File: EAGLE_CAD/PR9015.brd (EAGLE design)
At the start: 70 x 70 mm, 73 parts, among them J1 M3_SCREW_POST, SW1 C&K_PTS645

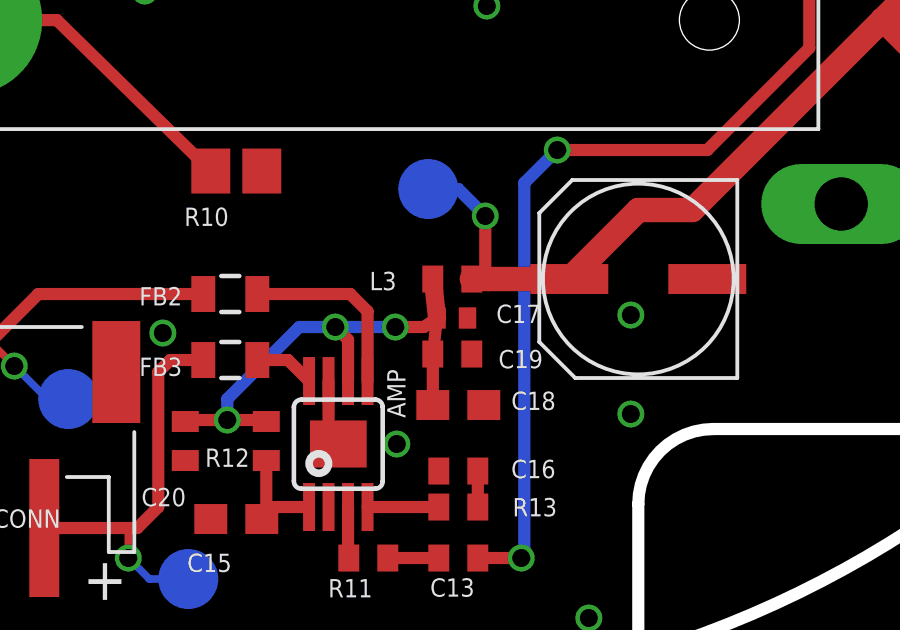
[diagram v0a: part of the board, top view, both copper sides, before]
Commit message: Revert cea9e40..4e97d22
This rolls back to commit cea9e40d509ff5bb8dd7e4369702d55ec1f1bc0f.
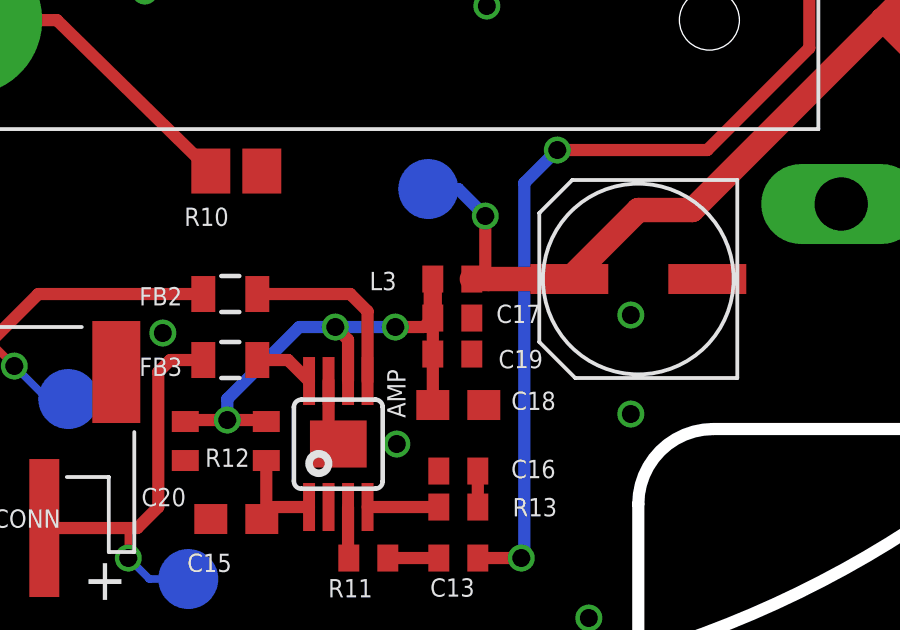
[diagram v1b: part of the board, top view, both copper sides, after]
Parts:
- C17: device PR_Parts_Library:C0402 -> resistor:C0402
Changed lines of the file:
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@@
 <?xml version="1.0" encoding="utf-8"?>
 <!DOCTYPE eagle SYSTEM "eagle.dtd">
-<eagle version="6.6.0">
+<eagle version="7.2.0">
 <drawing>
 <settings>
@@
 <setting verticaltext="up"/>
 </settings>
-<grid distance="0.1" unitdist="mm" unit="mm" style="lines" multiple="1" display="yes" altdistance="0.025" altunitdist="inch" altunit="inch"/>
+<grid distance="1" unitdist="mil" unit="mm" style="lines" multiple="1" display="yes" altdistance="0.025" altunitdist="inch" altunit="inch"/>
 <layers>
 <layer number="1" name="Top" color="4" fill="1" visible="yes" active="yes"/>
@@
 <pass name="Default">
 <param name="RoutingGrid" value="50mil"/>
+<param name="AutoGrid" value="1"/>
+<param name="Efforts" value="0"/>
+<param name="TopRouterVariant" value="1"/>
 <param name="tpViaShape" value="round"/>
 <param name="PrefDir.1" value="|"/>
@@
 <attribute name="VALUE" x="32.235" y="7.905" size="1.27" layer="27" rot="R180"/>
 </element>
-<element name="C17" library="PR_Parts_Library" package="C0402" value="1uf" x="38.8" y="12.7" smashed="yes" rot="R180">
+<element name="C17" library="resistor" package="C0402" value="1uf" x="38.8" y="12.7" smashed="yes" rot="R180">
 <attribute name="NAME" x="40.265" y="12.535" size="0.6096" layer="25" ratio="16"/>
 <attribute name="VALUE" x="39.435" y="14.605" size="1.27" layer="27" rot="R180"/>
@@
 <wire x1="34.9" y1="12.4" x2="33.7" y2="12.4" width="0.4064" layer="16"/>
 <wire x1="33.7" y1="12.4" x2="31.3" y2="10" width="0.4064" layer="16"/>
-<wire x1="38.2929" y1="12.7" x2="37.85" y2="12.4" width="0.4064" layer="1"/>
+<wire x1="38.15" y1="12.7" x2="37.85" y2="12.4" width="0.4064" layer="1"/>
 <wire x1="37.85" y1="12.4" x2="36.9" y2="12.4" width="0.4064" layer="1"/>
 <via x="36.9" y="12.4" extent="1-16" drill="0.6"/>
 <wire x1="36.9" y1="12.4" x2="34.9" y2="12.4" width="0.4064" layer="16"/>
 <wire x1="38.15" y1="9.8" x2="38.15" y2="11.5" width="0.4064" layer="1"/>
-<wire x1="38.15" y1="11.5" x2="38.2929" y2="12.7" width="0.4064" layer="1"/>
+<wire x1="38.15" y1="11.5" x2="38.15" y2="12.7" width="0.4064" layer="1"/>
 <wire x1="31.3" y1="10" x2="31.3" y2="9.3" width="0.4064" layer="16"/>
 <via x="31.3" y="9.3" extent="1-16" drill="0.6" diameter="0.4064"/>
@@
 <wire x1="31.3" y1="9.3" x2="29.95" y2="9.3" width="0.4064" layer="1"/>
 <wire x1="29.95" y1="9.3" x2="29.9" y2="9.25" width="0.4064" layer="1"/>
-<wire x1="38.2929" y1="12.7" x2="38.15" y2="14" width="0.6096" layer="1"/>
+<wire x1="38.15" y1="12.7" x2="38.15" y2="14" width="0.6096" layer="1"/>
 </signal>
 <signal name="N$20">
